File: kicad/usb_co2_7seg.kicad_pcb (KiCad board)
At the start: 2 copper layers, 95 x 72 mm, 16 parts, among them U1 PinHeader_XIAO, U2 PinHeader_XIAO, U3 SeeeduinoXIAO, U4 MH-Z19B, U5 TM1637, U6 7segment_led, U7 SW_push_2pin

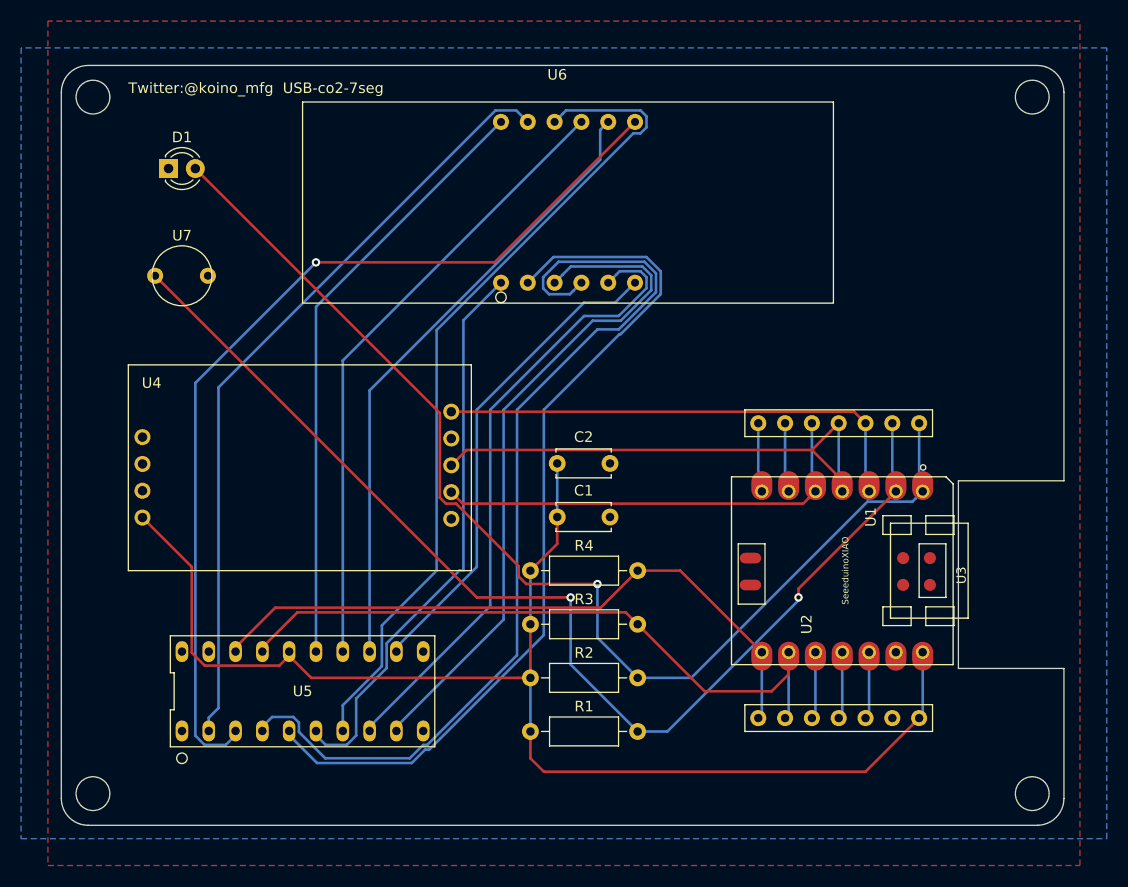
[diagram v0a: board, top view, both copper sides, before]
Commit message: 部品の仮置き
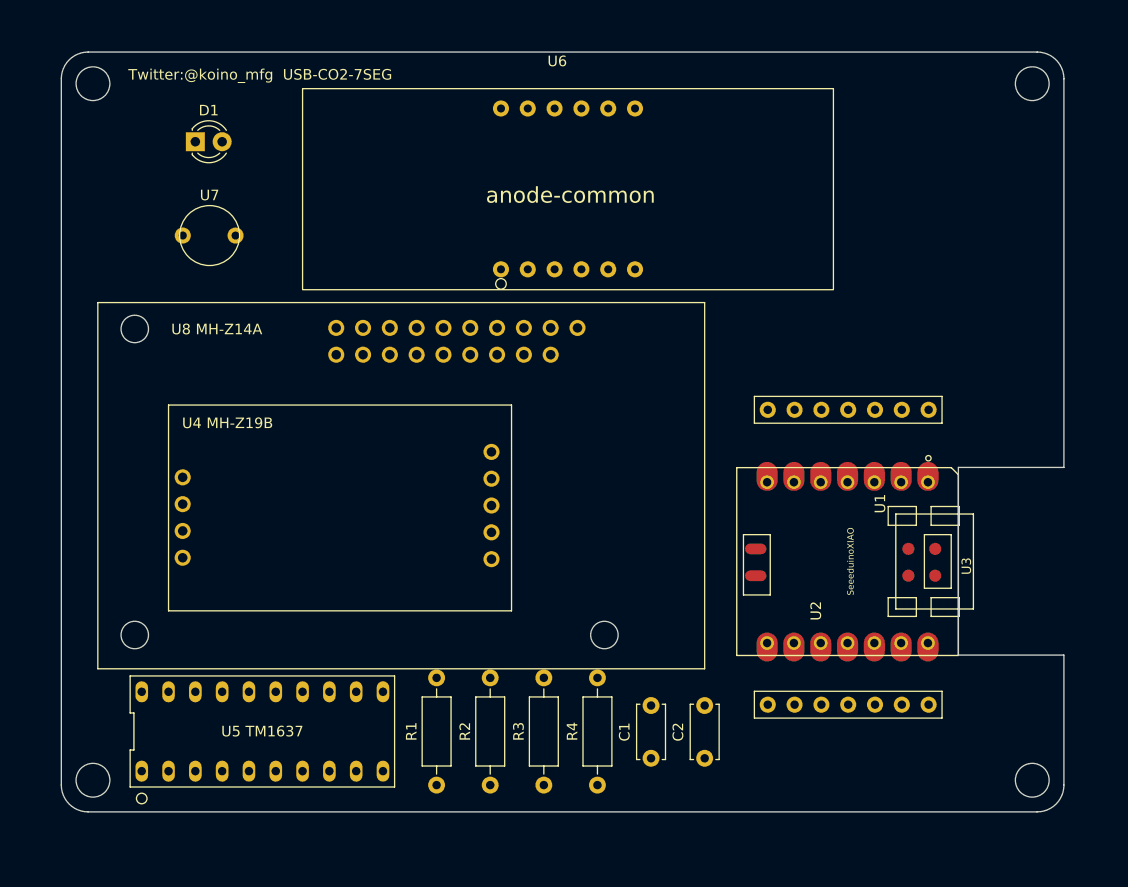
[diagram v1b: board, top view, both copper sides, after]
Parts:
- removed U4: MH-Z19B, kicad_mylib:MH-Z19B
- removed U5: TM1637, kicad_mylib:TM1630
- added U4 MH-Z19B: MH-Z19B, kicad_mylib:MH-Z19B, F.Cu at (10.2, -20.3)
- added U5 TM1637: TM1637, kicad_mylib:TM1630, F.Cu at (6.35, -3.81)
- added U8 MH-Z14A: MH-Z14A, kicad_mylib:MH-Z14A, F.Cu at (61.0, -49.5)
- moved C2 31.2 mm to (61.0, -6.35), turned to 90 degrees
- moved C1 24.5 mm to (55.9, -6.35), turned to 90 degrees
- moved R4 21.3 mm to (50.8, -3.81), turned to 90 degrees
- moved R3 15.3 mm to (45.7, -3.81), turned to 90 degrees
- moved R2 10.9 mm to (40.6, -3.81), turned to 90 degrees
- moved R1 10.2 mm to (35.6, -3.81), turned to 90 degrees
- moved U7 4.62 mm to (11.5, -55.9)
- moved D1 3.59 mm to (12.7, -64.8)
- moved U1 1.56 mm to (83.5, -38.1)
- moved U2 1.56 mm to (65.7, -12.7)
- moved ~ 1.27 mm to (0.00, -1.27)
- moved U6 1.27 mm to (22.9, -50.8)
- moved ~ 1.27 mm to (6.35, -69.8)
- moved U3 1.00 mm to (64.0, -33.9)
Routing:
- net +5V: track 123.8 -> 0.00 mm
- net Net-(D1-Pad2): track 111.1 -> 0.00 mm, vias 1 -> 0
- net Net-(R1-Pad2): track 108.8 -> 0.00 mm, vias 2 -> 0
- net Net-(U5-Pad4): track 91.0 -> 0.00 mm
- net Net-(U5-Pad3): track 90.3 -> 0.00 mm, vias 1 -> 0
- net Net-(U5-Pad5): track 83.9 -> 0.00 mm
- net Net-(U5-Pad7): track 79.9 -> 0.00 mm
- net Net-(U5-Pad2): track 73.6 -> 0.00 mm
- net Net-(U5-Pad9): track 64.9 -> 0.00 mm
- net Net-(R3-Pad2): track 63.5 -> 0.00 mm
- net Net-(R4-Pad2): track 62.9 -> 0.00 mm
- net Net-(U5-Pad8): track 60.1 -> 0.00 mm
- net Net-(U5-Pad14): track 59.6 -> 0.00 mm
- net Net-(U5-Pad13): track 59.6 -> 0.00 mm
- net Net-(U5-Pad15): track 57.5 -> 0.00 mm
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- removed copper zone on B.Cu, net GND
- removed copper zone on F.Cu, net GND
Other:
- board text added: "anode-common"
